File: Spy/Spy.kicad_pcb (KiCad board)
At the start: 2 copper layers, 8 parts, among them J1 Screw_Terminal_01x02, J2 Screw_Terminal_01x02, U1 ESP32-DevKitC, U2 GP2Y0A21YK0F, U3 GP2Y0A21YK0F, U4 SEN-12787, U5 L298N, U6 QTR-8A

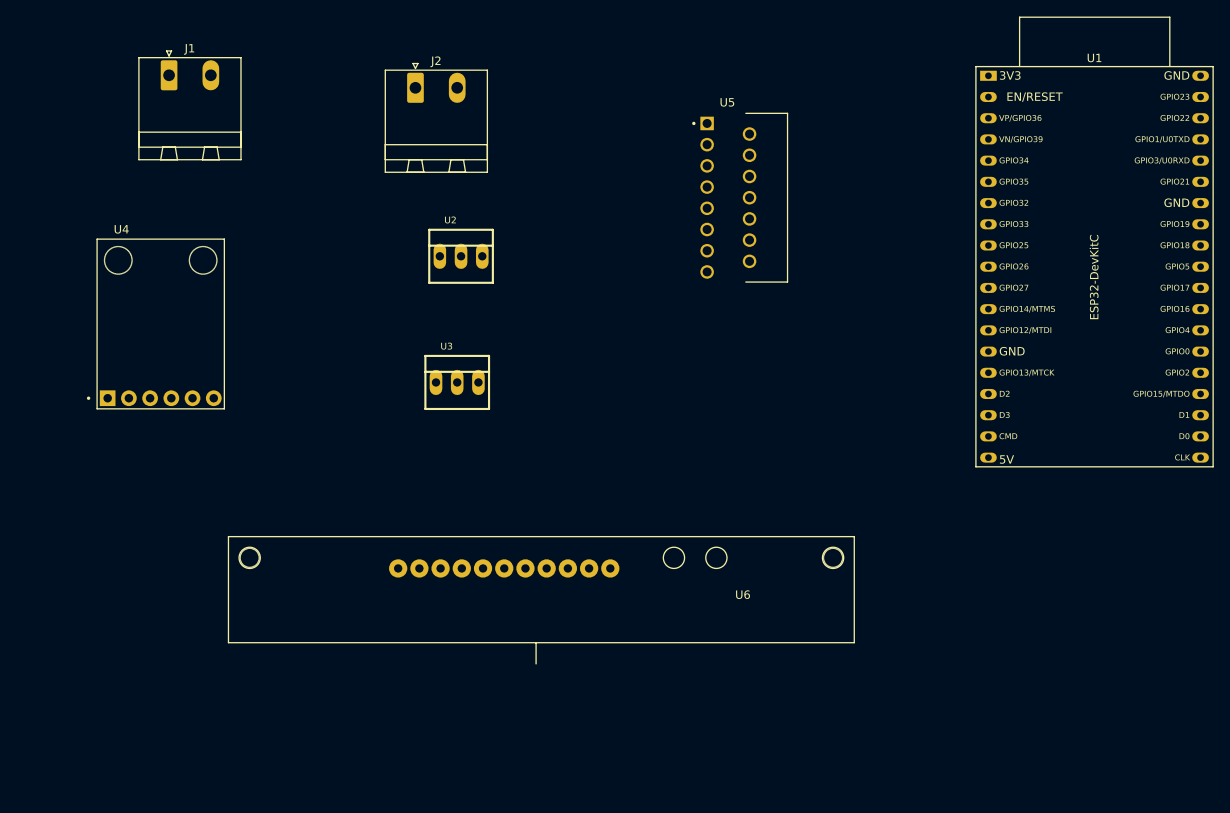
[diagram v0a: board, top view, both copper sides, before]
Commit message: pcb edited
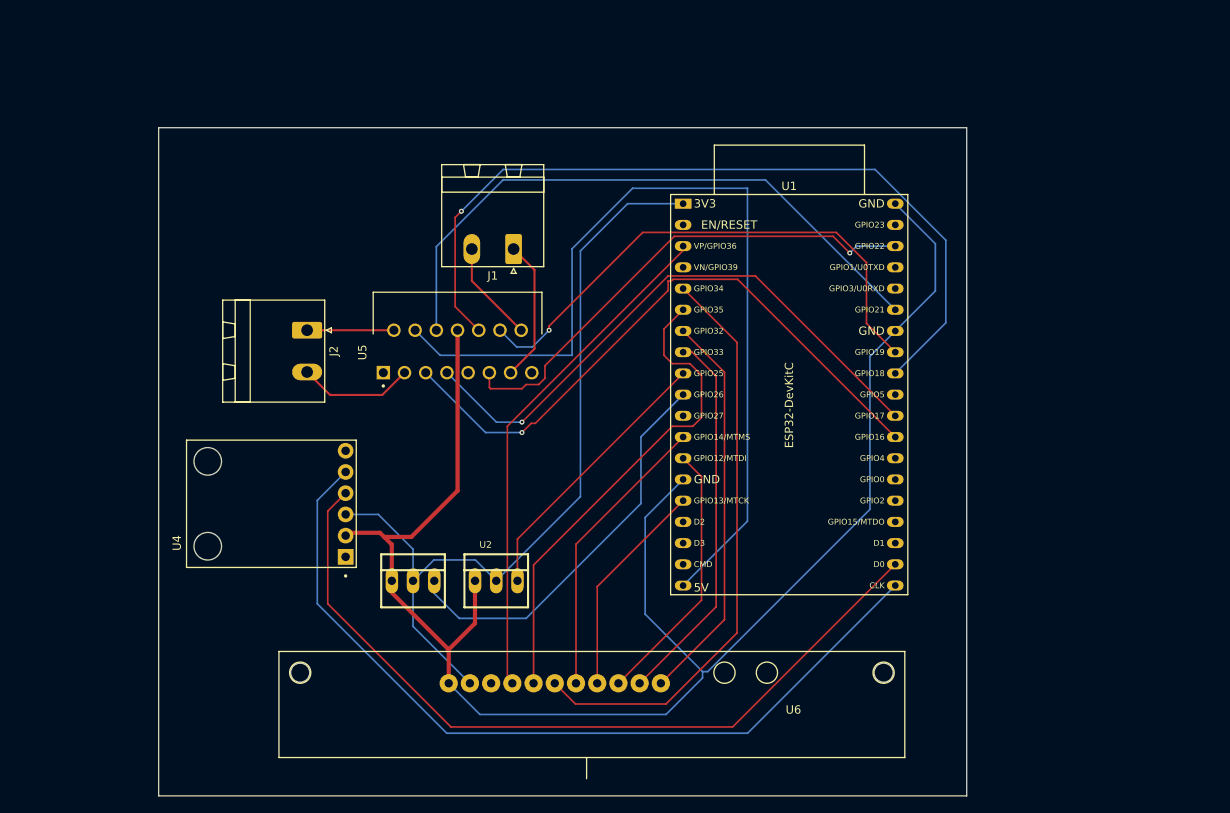
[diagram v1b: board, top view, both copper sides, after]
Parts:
- moved U5 48.9 mm to (94.2, 100.8), turned to 90 degrees
- moved J1 46.2 mm to (109.8, 86.0), turned to 180 degrees
- moved U1 39.6 mm to (130.1, 80.6)
- moved U2 39.1 mm to (107.7, 125.8)
- moved J2 31.8 mm to (85.0, 95.8), turned to -90 degrees
- moved U4 25.3 mm to (80.8, 116.5), turned to 90 degrees
- moved U3 24.3 mm to (97.7, 125.8)
- moved U6 15.0 mm to (135.0, 136.8)
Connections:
- J1 pad 1: unconnected-(J1-Pin_1-Pad1) -> Net-(J1-Pin_1)
- J1 pad 2: unconnected-(J1-Pin_2-Pad2) -> Net-(J1-Pin_2)
- J2 pad 1: unconnected-(J2-Pin_1-Pad1) -> Net-(J2-Pin_1)
- J2 pad 2: unconnected-(J2-Pin_2-Pad2) -> Net-(J2-Pin_2)
- U1 pad 1: unconnected-(U1-3V3-Pad1) -> Net-(U1-3V3)
- U1 pad 10: unconnected-(U1-DAC_2/ADC2_CH9/GPIO26-Pad10) -> Net-(U1-DAC_2/ADC2_CH9/GPIO26)
- U1 pad 12: unconnected-(U1-MTMS/GPIO14/ADC2_CH6-Pad12) -> Net-(U1-MTMS/GPIO14/ADC2_CH6)
- U1 pad 13: unconnected-(U1-MTDI/GPIO12/ADC2_CH5-Pad13) -> Net-(U1-MTDI/GPIO12/ADC2_CH5)
- U1 pad 14: Net-(U1-GND-Pad14) -> GND
- U1 pad 15: unconnected-(U1-MTCK/GPIO13/ADC2_CH4-Pad15) -> Net-(U1-MTCK/GPIO13/ADC2_CH4)
- U1 pad 19: unconnected-(U1-5V-Pad19) -> Net-(U1-5V)
- U1 pad 20: unconnected-(U1-SD_CLK/GPIO6-Pad20) -> Net-(U1-SD_CLK/GPIO6)
- U1 pad 21: unconnected-(U1-SD_DATA0/GPIO7-Pad21) -> Net-(U1-SD_DATA0/GPIO7)
- U1 pad 27: unconnected-(U1-GPIO16-Pad27) -> Net-(U1-GPIO16)
- U1 pad 28: unconnected-(U1-GPIO17-Pad28) -> Net-(U1-GPIO17)
- U1 pad 3: unconnected-(U1-SENSOR_VP/GPIO36/ADC1_CH0-Pad3) -> Net-(U1-SENSOR_VP/GPIO36/ADC1_CH0)
- U1 pad 30: unconnected-(U1-GPIO18-Pad30) -> Net-(U1-GPIO18)
- U1 pad 31: unconnected-(U1-GPIO19-Pad31) -> Net-(U1-GPIO19)
- U1 pad 32: Net-(U1-GND-Pad14) -> GND
- U1 pad 33: unconnected-(U1-GPIO21-Pad33) -> Net-(U1-GPIO21)
- U1 pad 36: unconnected-(U1-GPIO22-Pad36) -> Net-(U1-GPIO22)
- U1 pad 38: Net-(U1-GND-Pad14) -> GND
- U1 pad 5: unconnected-(U1-VDET_1/GPIO34/ADC1_CH6-Pad5) -> Net-(U1-VDET_1/GPIO34/ADC1_CH6)
- U1 pad 6: unconnected-(U1-VDET_2/GPIO35/ADC1_CH7-Pad6) -> Net-(U1-VDET_2/GPIO35/ADC1_CH7)
- U1 pad 7: unconnected-(U1-32K_XP/GPIO32/ADC1_CH4-Pad7) -> Net-(U1-32K_XP/GPIO32/ADC1_CH4)
- U1 pad 8: unconnected-(U1-32K_XN/GPIO33/ADC1_CH5-Pad8) -> Net-(U1-32K_XN/GPIO33/ADC1_CH5)
- U1 pad 9: unconnected-(U1-DAC_1/ADC2_CH8/GPIO25-Pad9) -> Net-(U1-DAC_1/ADC2_CH8/GPIO25)
- U2 pad 1: unconnected-(U2-GND-Pad1) -> GND
- U2 pad 2: unconnected-(U2-VCC-Pad2) -> Net-(U1-3V3)
- U2 pad 3: unconnected-(U2-VOUT-Pad3) -> Net-(U1-DAC_1/ADC2_CH8/GPIO25)
- U3 pad 1: unconnected-(U3-GND-Pad1) -> GND
- U3 pad 2: unconnected-(U3-VCC-Pad2) -> Net-(U1-3V3)
- U3 pad 3: unconnected-(U3-VOUT-Pad3) -> Net-(U1-DAC_2/ADC2_CH9/GPIO26)
- U4 pad 2: unconnected-(U4-GND-Pad2) -> GND
- U4 pad 3: unconnected-(U4-VCC-Pad3) -> Net-(U1-3V3)
- U4 pad 4: unconnected-(U4-SDA-Pad4) -> Net-(U1-SD_DATA0/GPIO7)
- U4 pad 5: unconnected-(U4-SCL-Pad5) -> Net-(U1-SD_CLK/GPIO6)
- U5 pad 10: unconnected-(U5-IN3-Pad10) -> Net-(U1-GPIO18)
- U5 pad 11: unconnected-(U5-ENB-Pad11) -> Net-(U1-GPIO22)
- U5 pad 12: unconnected-(U5-IN4-Pad12) -> Net-(U1-GPIO19)
- U5 pad 13: unconnected-(U5-OUT3-Pad13) -> Net-(J1-Pin_1)
- U5 pad 14: unconnected-(U5-OUT4-Pad14) -> Net-(J1-Pin_2)
- U5 pad 2: unconnected-(U5-OUT1-Pad2) -> Net-(J2-Pin_1)
- U5 pad 3: unconnected-(U5-OUT2-Pad3) -> Net-(J2-Pin_2)
- U5 pad 4: unconnected-(U5-VS-Pad4) -> Net-(U1-5V)
- U5 pad 5: unconnected-(U5-IN1-Pad5) -> Net-(U1-GPIO16)
- U5 pad 6: unconnected-(U5-ENA-Pad6) -> Net-(U1-GPIO21)
- U5 pad 7: unconnected-(U5-IN2-Pad7) -> Net-(U1-GPIO17)
- U5 pad 8: unconnected-(U5-GND-Pad8) -> GND
- U5 pad 9: unconnected-(U5-VSS-Pad9) -> +12V
- U6 pad 3V3: unconnected-(U6-Pad3V3) -> Net-(U1-3V3)
- U6 pad GND: unconnected-(U6-PadGND) -> GND
- U6 pad LED1: unconnected-(U6-PadLED1) -> Net-(U1-SENSOR_VP/GPIO36/ADC1_CH0)
- U6 pad LED2: unconnected-(U6-PadLED2) -> Net-(U1-VDET_2/GPIO35/ADC1_CH7)
- U6 pad LED3: unconnected-(U6-PadLED3) -> Net-(U1-VDET_1/GPIO34/ADC1_CH6)
- U6 pad LED4: unconnected-(U6-PadLED4) -> Net-(U1-MTMS/GPIO14/ADC2_CH6)
- U6 pad LED5: unconnected-(U6-PadLED5) -> Net-(U1-MTCK/GPIO13/ADC2_CH4)
- U6 pad LED6: unconnected-(U6-PadLED6) -> Net-(U1-MTDI/GPIO12/ADC2_CH5)
- U6 pad LED7: unconnected-(U6-PadLED7) -> Net-(U1-32K_XN/GPIO33/ADC1_CH5)
- U6 pad LED8: unconnected-(U6-PadLED8) -> Net-(U1-32K_XP/GPIO32/ADC1_CH4)
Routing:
- net GND: track 0.00 -> 197.8 mm
- net Net-(U1-5V): track 0.00 -> 107.5 mm
- net Net-(U1-SD_CLK/GPIO6): track 0.00 -> 100.1 mm
- net Net-(U1-3V3): track 0.00 -> 99.0 mm
- net Net-(U1-GPIO18): track 0.00 -> 97.8 mm, vias 0 -> 1
- net Net-(U1-SD_DATA0/GPIO7): track 0.00 -> 96.3 mm
- net Net-(U1-GPIO16): track 0.00 -> 75.3 mm, vias 0 -> 1
- net Net-(U1-GPIO21): track 0.00 -> 74.7 mm
- net Net-(U1-GPIO17): track 0.00 -> 70.3 mm, vias 0 -> 1
- net Net-(U1-VDET_1/GPIO34/ADC1_CH6): track 0.00 -> 70.3 mm
- net Net-(U1-GPIO19): track 0.00 -> 64.3 mm, vias 0 -> 1
- net Net-(U1-SENSOR_VP/GPIO36/ADC1_CH0): track 0.00 -> 61.3 mm
- net Net-(U1-GPIO22): track 0.00 -> 60.0 mm, vias 0 -> 1
- net Net-(U1-VDET_2/GPIO35/ADC1_CH7): track 0.00 -> 58.5 mm
- net Net-(U1-DAC_2/ADC2_CH9/GPIO26): track 0.00 -> 48.3 mm
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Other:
- board outline added: 96.8 x 80 mm

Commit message: new pcb
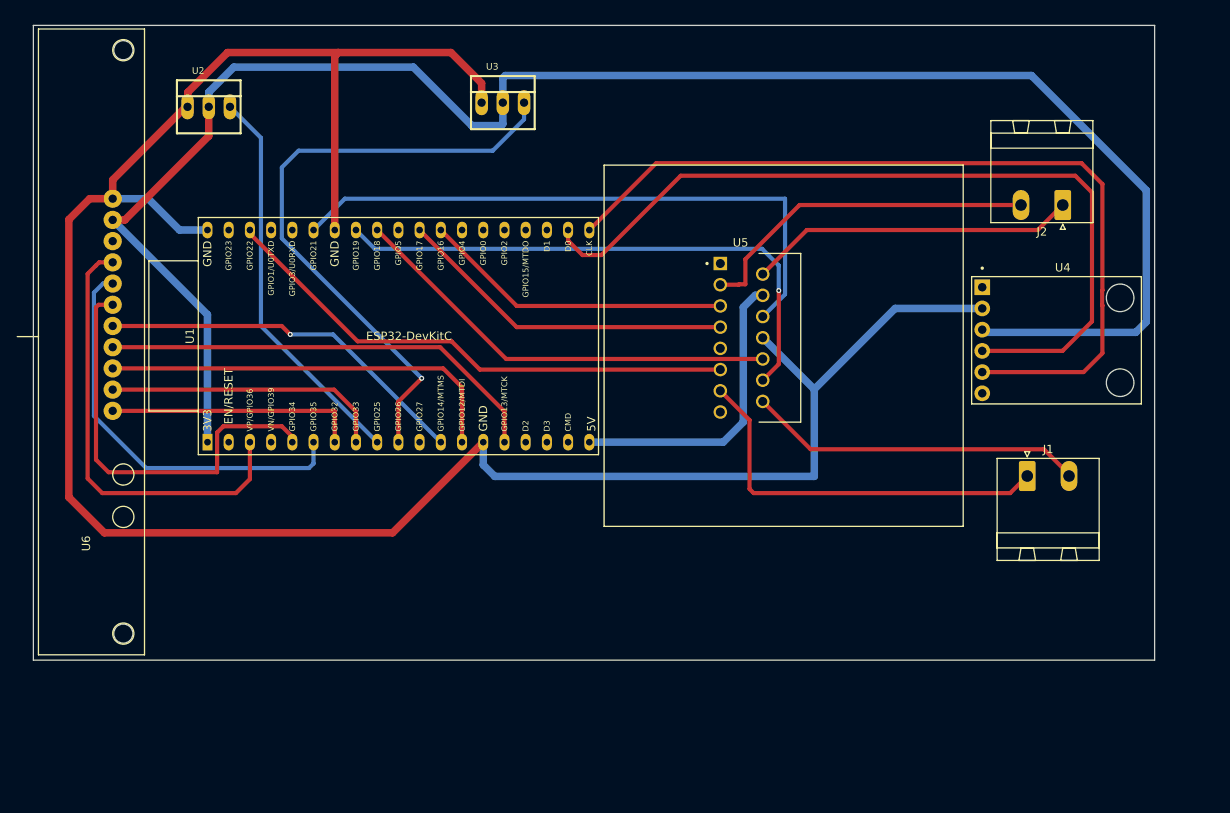
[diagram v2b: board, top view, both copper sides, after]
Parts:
- moved U4 96.0 mm to (174.8, 97.0), turned to -90 degrees
- moved J2 91.7 mm to (175.5, 80.8), turned to 180 degrees
- moved U6 75.8 mm to (63.0, 113.0), turned to -90 degrees
- moved J1 67.2 mm to (171.2, 113.2), turned to 0 degrees
- moved U2 66.4 mm to (73.2, 69.0)
- moved U1 63.7 mm to (73.1, 109.2), turned to 90 degrees
- moved U3 58.3 mm to (108.5, 68.5)
- moved U5 42.4 mm to (134.5, 87.8), turned to 0 degrees
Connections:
- net Net-(U1-32K_XN/GPIO33/ADC1_CH5) renamed GPIO33
- net Net-(U1-32K_XP/GPIO32/ADC1_CH4) renamed GPIO32
- net Net-(U1-3V3) renamed 3V3
- net Net-(U1-DAC_1/ADC2_CH8/GPIO25) renamed GPIO25
- net Net-(U1-DAC_2/ADC2_CH9/GPIO26) renamed GPIO26
- net Net-(U1-GPIO16) renamed GPIO16
- net Net-(U1-GPIO17) renamed GPIO17
- net Net-(U1-GPIO18) renamed GPIO18
- net Net-(U1-GPIO19) renamed GPIO19
- net Net-(U1-GPIO21) renamed GPIO21
- net Net-(U1-GPIO22) renamed GPIO22
- net Net-(U1-MTCK/GPIO13/ADC2_CH4) renamed GPIO13
- net Net-(U1-MTDI/GPIO12/ADC2_CH5) renamed GPIO12
- net Net-(U1-MTMS/GPIO14/ADC2_CH6) renamed GPIO14
- net Net-(U1-SD_CLK/GPIO6) renamed GPIO6
- net Net-(U1-SD_DATA0/GPIO7) renamed GPIO7
- net Net-(U1-SENSOR_VP/GPIO36/ADC1_CH0) renamed GPIO36
- net Net-(U1-VDET_1/GPIO34/ADC1_CH6) renamed GPIO34
- net Net-(U1-VDET_2/GPIO35/ADC1_CH7) renamed GPIO35
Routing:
- net 3V3: track 99.0 -> 216.1 mm
- net GND: track 197.8 -> 273.7 mm
- net Net-(U1-5V): track 107.5 -> 36.1 mm
- net GPIO18: track 97.8 -> 52.6 mm, vias 1 -> 0
- net GPIO16: track 75.3 -> 37.2 mm, vias 1 -> 0
- net Net-(J1-Pin_1): track 17.0 -> 47.5 mm
- net GPIO17: track 70.3 -> 40.8 mm, vias 1 -> 0
- net Net-(J2-Pin_1): track 10.4 -> 39.3 mm
- net Net-(J1-Pin_2): track 12.2 -> 40.5 mm
- net Net-(J2-Pin_2): track 13.9 -> 41.7 mm
- net GPIO13: track 26.1 -> 53.8 mm
- net GPIO26: track 48.3 -> 74.4 mm, vias 0 -> 1
- net GPIO34: track 70.3 -> 50.7 mm
- net GPIO12: track 32.0 -> 49.3 mm
- net GPIO32: track 47.4 -> 30.3 mm
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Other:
- board size 96.8 x 80 mm -> 134.2 x 76 mm
